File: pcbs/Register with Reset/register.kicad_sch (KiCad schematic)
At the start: 28 parts, among them U301 74HC245, U302 74HCT574, U303 74HC245

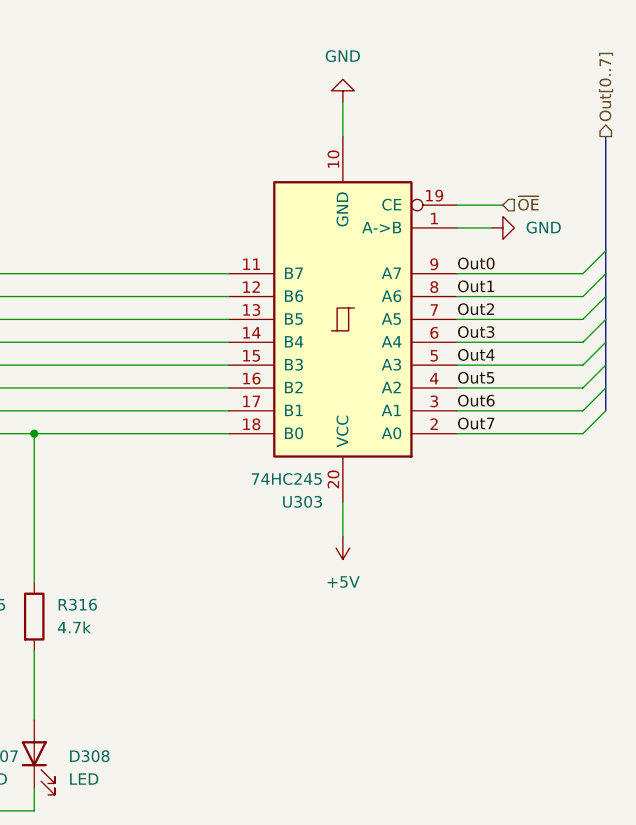
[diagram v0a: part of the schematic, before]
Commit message: Get buses routed
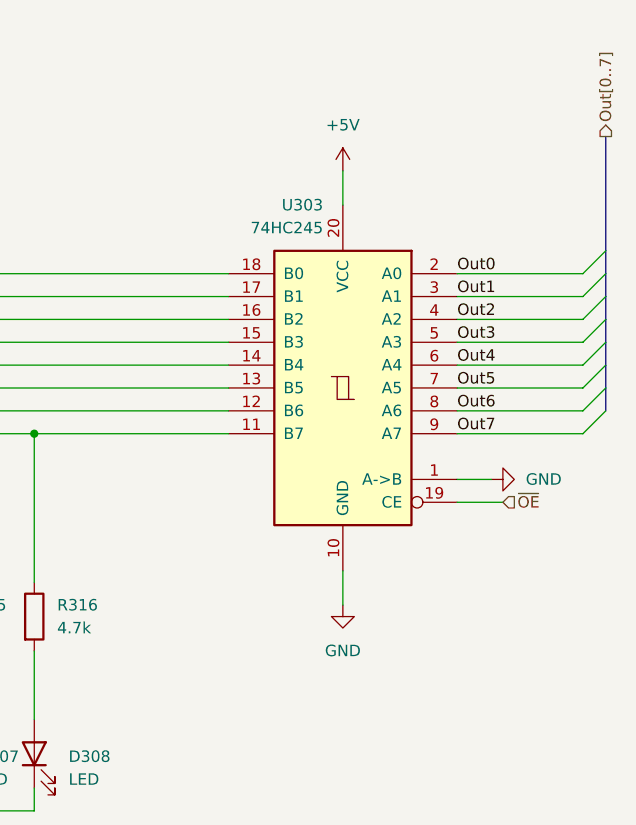
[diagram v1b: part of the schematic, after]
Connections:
- net Out0: now also U303.2 (A0); no longer U303.9 (A7)
- net Out1: now also U303.3 (A1); no longer U303.8 (A6)
- net Out2: now also U303.4 (A2); no longer U303.7 (A5)
- net Out3: now also U303.5 (A3); no longer U303.6 (A4)
- net Out4: now also U303.6 (A4); no longer U303.5 (A3)
- net Out5: now also U303.7 (A5); no longer U303.4 (A2)
- net Out6: now also U303.8 (A6); no longer U303.3 (A1)
- net Out7: now also U303.9 (A7); no longer U303.2 (A0)
- net at R314.1, U302.14 (Q5): now also U303.13 (B5); no longer U303.16 (B2)
- net at R316.1, U302.12 (Q7): now also U303.11 (B7); no longer U303.18 (B0)
- net at R315.1, U302.13 (Q6): now also U303.12 (B6); no longer U303.17 (B1)
- net at R313.1, U302.15 (Q4): now also U303.14 (B4); no longer U303.15 (B3)
- net at R312.1, U302.16 (Q3): now also U303.15 (B3); no longer U303.14 (B4)
- net at R311.1, U302.17 (Q2): now also U303.16 (B2); no longer U303.13 (B5)
- net at R310.1, U302.18 (Q1): now also U303.17 (B1); no longer U303.12 (B6)
- net at R309.1, U302.19 (Q0): now also U303.18 (B0); no longer U303.11 (B7)
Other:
- moved on the sheet: U303
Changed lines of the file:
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@@
 	(wire
 		(pts
-			(xy 264.16 34.29) (xy 269.24 34.29)
+			(xy 264.16 67.31) (xy 269.24 67.31)
 		)
 		(stroke
@@
 	(wire
 		(pts
-			(xy 251.46 22.86) (xy 251.46 26.67)
+			(xy 251.46 78.74) (xy 251.46 74.93)
 		)
 		(stroke
@@
 	(wire
 		(pts
-			(xy 251.46 67.31) (xy 251.46 71.12)
+			(xy 251.46 34.29) (xy 251.46 30.48)
 		)
 		(stroke
@@
 	(wire
 		(pts
-			(xy 264.16 36.83) (xy 267.97 36.83)
+			(xy 264.16 64.77) (xy 267.97 64.77)
 		)
 		(stroke
@@
 	(hierarchical_label "~{OE}"
 		(shape input)
-		(at 269.24 34.29 0)
+		(at 269.24 67.31 0)
 		(fields_autoplaced yes)
 		(effects
@@
 	(symbol
 		(lib_id "power:GND")
-		(at 251.46 22.86 180)
+		(at 251.46 78.74 0)
 		(unit 1)
 		(exclude_from_sim no)
@@
 		(fields_autoplaced yes)
 		(property "Reference" "#PWR0312"
-			(at 251.46 16.51 0)
+			(at 251.46 85.09 0)
 			(effects
 				(font
@@
 		)
 		(property "Value" "GND"
-			(at 251.46 17.78 0)
+			(at 251.46 83.82 0)
 			(effects
 				(font
@@
 		)
 		(property "Footprint" ""
-			(at 251.46 22.86 0)
+			(at 251.46 78.74 0)
 			(effects
 				(font
@@
 		)
 		(property "Datasheet" ""
-			(at 251.46 22.86 0)
+			(at 251.46 78.74 0)
 			(effects
 				(font
@@
 		)
 		(property "Description" "Power symbol creates a global label with name \"GND\" , ground"
-			(at 251.46 22.86 0)
+			(at 251.46 78.74 0)
 			(effects
 				(font
@@
 	(symbol
 		(lib_id "power:+5V")
-		(at 251.46 71.12 180)
+		(at 251.46 30.48 0)
 		(unit 1)
 		(exclude_from_sim no)
@@
 		(fields_autoplaced yes)
 		(property "Reference" "#PWR0311"
-			(at 251.46 67.31 0)
+			(at 251.46 34.29 0)
 			(effects
 				(font
@@
 		)
 		(property "Value" "+5V"
-			(at 251.46 76.2 0)
+			(at 251.46 25.4 0)
 			(effects
 				(font
@@
 		)
 		(property "Footprint" ""
-			(at 251.46 71.12 0)
+			(at 251.46 30.48 0)
 			(effects
 				(font
@@
 		)
 		(property "Datasheet" ""
-			(at 251.46 71.12 0)
+			(at 251.46 30.48 0)
 			(effects
 				(font
@@
 		)
 		(property "Description" "Power symbol creates a global label with name \"+5V\""
-			(at 251.46 71.12 0)
+			(at 251.46 30.48 0)
 			(effects
 				(font
@@
 	(symbol
 		(lib_id "power:GND")
-		(at 267.97 36.83 90)
+		(at 267.97 64.77 90)
 		(unit 1)
 		(exclude_from_sim no)
@@
 		(fields_autoplaced yes)
 		(property "Reference" "#PWR0310"
-			(at 274.32 36.83 0)
+			(at 274.32 64.77 0)
 			(effects
 				(font
@@
 		)
 		(property "Value" "GND"
-			(at 271.78 36.8299 90)
+			(at 271.78 64.7699 90)
 			(effects
 				(font
@@
 		)
 		(property "Footprint" ""
-			(at 267.97 36.83 0)
+			(at 267.97 64.77 0)
 			(effects
 				(font
@@
 		)
 		(property "Datasheet" ""
-			(at 267.97 36.83 0)
+			(at 267.97 64.77 0)
 			(effects
 				(font
@@
 		)
 		(property "Description" "Power symbol creates a global label with name \"GND\" , ground"
-			(at 267.97 36.83 0)
+			(at 267.97 64.77 0)
 			(effects
 				(font
@@
 	(symbol
 		(lib_id "74xx:74HC245")
-		(at 251.46 46.99 180)
+		(at 251.46 54.61 0)
+		(mirror y)
 		(unit 1)
 		(exclude_from_sim no)
@@
 		(dnp no)
 		(property "Reference" "U303"
-			(at 249.2659 67.31 0)
+			(at 249.2659 34.29 0)
 			(effects
 				(font
@@
 		)
 		(property "Value" "74HC245"
-			(at 249.2659 64.77 0)
+			(at 249.2659 36.83 0)
 			(effects
 				(font
@@
 		)
 		(property "Footprint" "Package_SO:SOIC-20W_7.5x12.8mm_P1.27mm"
-			(at 251.46 46.99 0)
+			(at 251.46 54.61 0)
 			(effects
 				(font
@@
 		)
 		(property "Datasheet" "http://www.ti.com/lit/gpn/sn74HC245"
-			(at 251.46 46.99 0)
+			(at 251.46 54.61 0)
 			(effects
 				(font
@@
 		)
 		(property "Description" "Octal BUS Transceivers, 3-State outputs"
-			(at 251.46 46.99 0)
+			(at 251.46 54.61 0)
 			(effects
 				(font
@@
 		)
 		(property "LCSC" "C5625"
-			(at 251.46 46.99 0)
+			(at 251.46 54.61 0)
 			(effects
 				(font
